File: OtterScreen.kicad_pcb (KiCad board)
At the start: 2 copper layers, 44.8 x 31.4 mm, 27 parts, among them J1 47272-0001, J2 USB-C_Power, U1 5022505191, U2 NE555, U3 DIO5661, U4 DIO5661

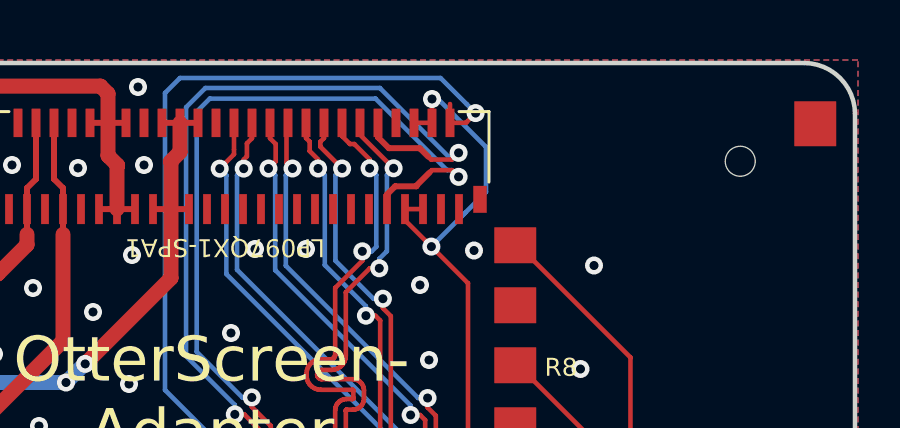
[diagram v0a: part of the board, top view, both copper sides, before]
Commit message: updated files
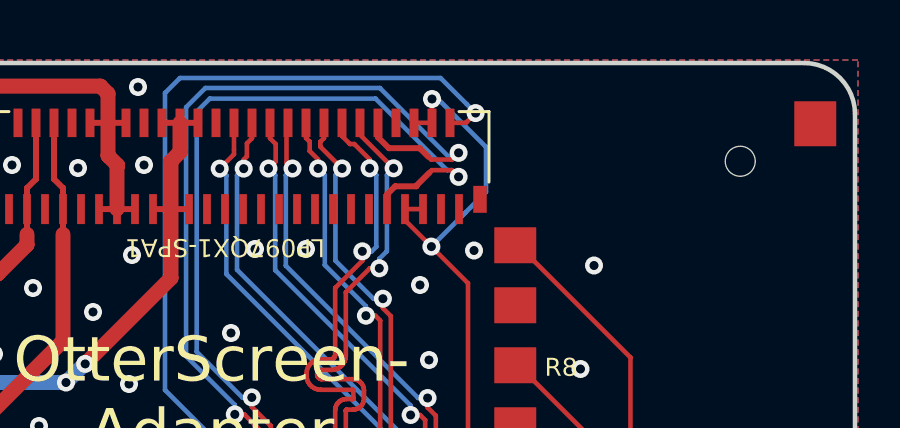
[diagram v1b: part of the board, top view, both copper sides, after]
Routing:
- net HPD: track 30.4 -> 29.7 mm
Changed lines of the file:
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@@
-(kicad_pcb (version 20171130) (host pcbnew 5.1.2)
+(kicad_pcb (version 20171130) (host pcbnew 5.0.1)
   (general
     (thickness 1.6)
     (drawings 15)
-    (tracks 718)
+    (tracks 717)
     (zones 0)
     (modules 27)
@@
     (zone_45_only no)
     (trace_min 0.154)
+    (segment_width 0.2)
+    (edge_width 0.15)
     (via_size 0.6)
     (via_drill 0.3)
@@
     (uvia_min_size 0.2)
     (uvia_min_drill 0.1)
-    (edge_width 0.15)
-    (segment_width 0.2)
     (pcb_text_width 0.3)
     (pcb_text_size 1.5 1.5)
@@
     (uvia_dia 0.3)
     (uvia_drill 0.1)
+    (diff_pair_gap 0.2)
     (diff_pair_width 0.154)
-    (diff_pair_gap 0.2)
     (add_net +3V3)
     (add_net +5V)
@@
   (via (at 145.1 127.4) (size 0.6) (drill 0.3) (layers F.Cu B.Cu) (net 3))
   (segment (start 145.15 127.45) (end 145.1 127.4) (width 0.154) (layer F.Cu) (net 3))
-  (segment (start 152.3 116.195) (end 152.3 115.566) (width 0.154) (layer F.Cu) (net 3))
   (segment (start 152.853894 116.168989) (end 153.153893 115.86899) (width 0.154) (layer F.Cu) (net 3))
   (segment (start 152.827883 116.195) (end 152.853894 116.168989) (width 0.154) (layer F.Cu) (net 3))

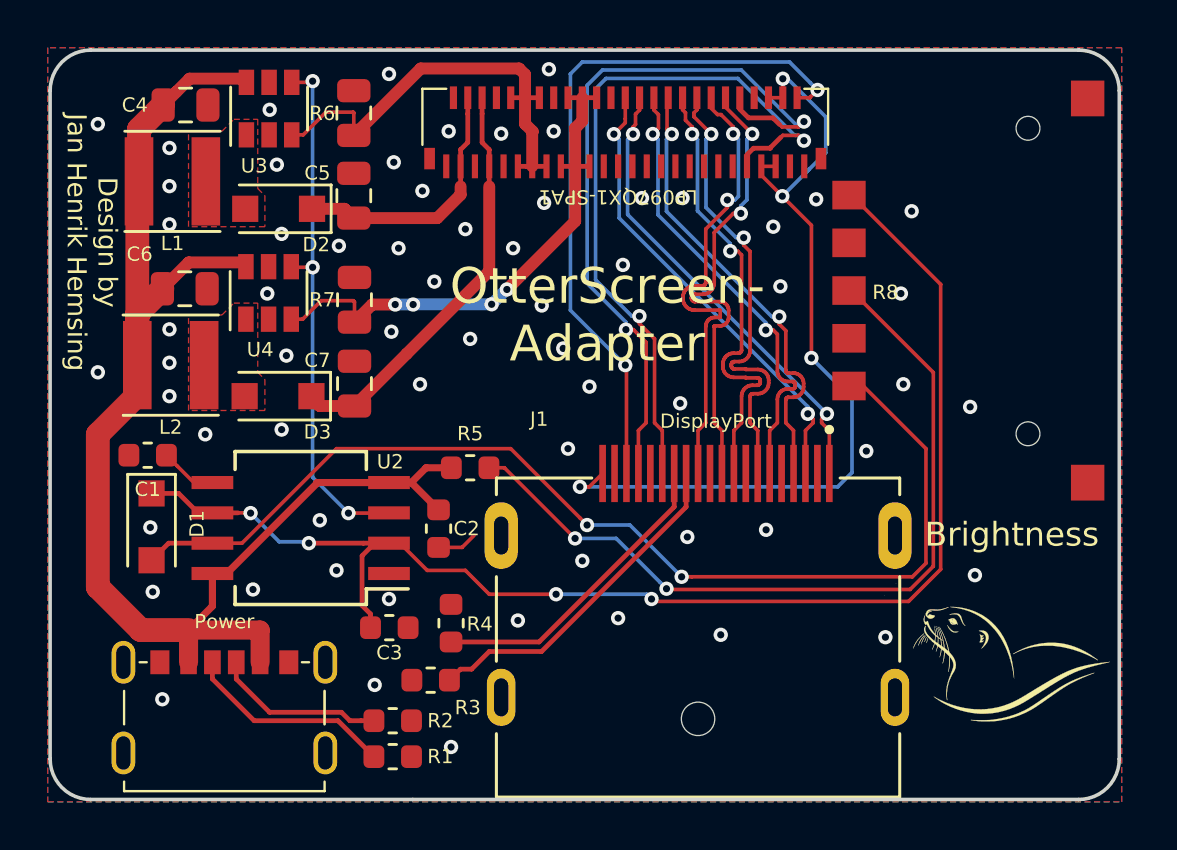
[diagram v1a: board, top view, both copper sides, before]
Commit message: fixed bugs, added ams1117
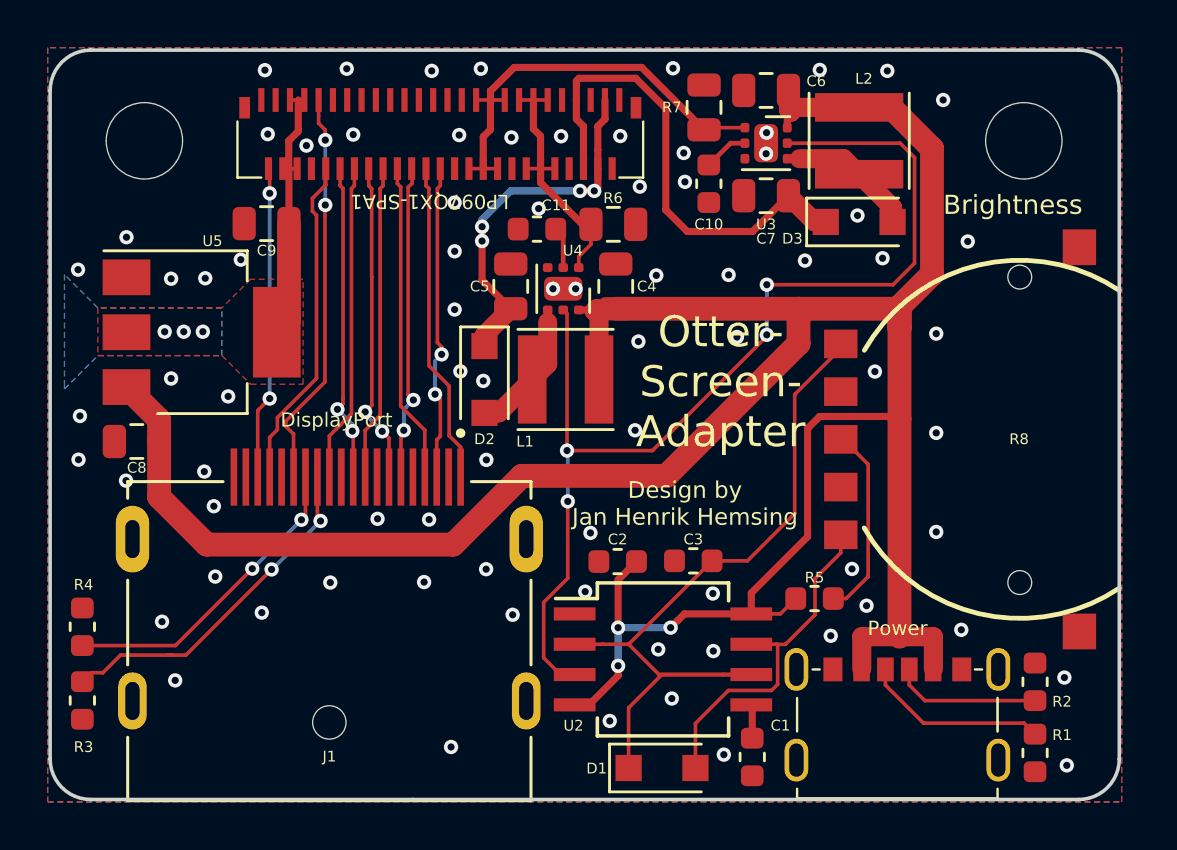
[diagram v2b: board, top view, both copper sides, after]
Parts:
- removed G***: LOGO, otter:otter_wave_118
- added C10: 220nF, Capacitor_SMD:C_0603_1608Metric, F.Cu at (148.6, 119.8)
- added C11: 220nF, Capacitor_SMD:C_0603_1608Metric, F.Cu at (141.4, 121.7)
- added C8: 0.47uF, Capacitor_SMD:C_0805_2012Metric, F.Cu at (124.6, 130.6)
- added C9: 0.47uF, Capacitor_SMD:C_0805_2012Metric, F.Cu at (130.1, 121.5)
- added H1: MountingHole_Pad, MountingHole:MountingHole_3.2mm_M3, F.Cu at (125.0, 118.0)
- added H2: MountingHole_Pad, MountingHole:MountingHole_3.2mm_M3, F.Cu at (161.8, 118.0)
- added U5: AMS1117-3.3, Package_TO_SOT_SMD:SOT-223-3_TabPin2, F.Cu at (127.3, 126.0)
- R6, R7: value R8 -> 0.8
- U3, U4: value DIO5661 -> TPS61160A; footprint Package_TO_SOT_SMD:SOT-23-6 -> Package_SON:WSON-6-1EP_2x2mm_P0.65mm_EP1x1.6mm
- moved L2 30.3 mm to (154.9, 118.0), turned to 270 degrees
- moved C1 28.3 mm to (150.4, 143.8), turned to 270 degrees
- moved J2 28.2 mm to (156.5, 140.2)
- moved R2 27.0 mm to (162.3, 140.7), turned to 90 degrees
- moved R1 26.9 mm to (162.3, 143.7), turned to 270 degrees
- moved C6 25.7 mm to (151.0, 115.9), turned to 180 degrees
- moved D3 25.4 mm to (154.9, 121.4), turned to 0 degrees
- moved D1 23.7 mm to (146.6, 144.3), turned to 0 degrees
- moved U3 20.9 mm to (151.0, 118.1), turned to 0 degrees
- moved C4 19.6 mm to (144.7, 124.1), turned to 90 degrees
- moved C7 19.0 mm to (151.0, 120.3), turned to 180 degrees
- moved L1 18.4 mm to (142.6, 128.0), turned to 180 degrees
- moved R7 16.7 mm to (148.4, 116.6)
- moved U2 16.1 mm to (146.7, 139.7), turned to 0 degrees
- moved J1 15.5 mm to (132.7, 145.7)
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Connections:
- J1 pad 20: +3V3 -> Net-(J1-Pad20)
- U3 pad 1: Net-(D2-Pad2) -> LEDC2
- U3 pad 2: GND -> Net-(C10-Pad1)
- U3 pad 3: LEDC1 -> GND
- U3 pad 4: PWM -> Net-(D3-Pad2)
- U3 pad 5: Net-(U3-Pad5) -> PWM
- U4 pad 1: Net-(D3-Pad2) -> LEDC1
- U4 pad 2: GND -> Net-(C11-Pad1)
- U4 pad 3: LEDC2 -> GND
- U4 pad 4: PWM -> Net-(D2-Pad2)
- U4 pad 5: Net-(U4-Pad5) -> PWM
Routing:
- net +5V: track 59.5 -> 120.1 mm, vias 0 -> 3
- net Net-(D1-Pad2): track 46.0 -> 14.8 mm, vias 2 -> 0
- net Net-(R5-Pad2): track 34.2 -> 8.12 mm, vias 2 -> 0
- net +3V3: track 36.0 -> 11.3 mm, vias 4 -> 3
- net Net-(C3-Pad1): track 57.3 -> 33.4 mm, vias 4 -> 0
- net PWM: track 22.2 -> 45.8 mm, vias 3 -> 4
- net AUX_N: track 31.6 -> 14.0 mm, vias 2 -> 0
- net HPD: track 29.7 -> 13.2 mm
- net AUX_P: track 30.8 -> 16.7 mm
- net LEDC1: track 18.8 -> 10.8 mm
- net L0_N: track 19.6 -> 13.3 mm
- net L0_P: track 19.6 -> 13.4 mm, vias 2 -> 0
- net L1_P: track 19.5 -> 13.2 mm, vias 2 -> 0
- net L1_N: track 19.7 -> 13.5 mm
- net L3_P: track 19.5 -> 13.4 mm
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- added copper zone on B.Cu, net +3V3
- added copper zone on F.Cu, net +3V3
- removed copper zone on F.Cu, net Net-(D2-Pad2)
- removed copper zone on F.Cu, net Net-(D3-Pad2)
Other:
- board text added: "Otter- Screen- Adapter"
- board text removed: "OtterScreen- Adapter"
